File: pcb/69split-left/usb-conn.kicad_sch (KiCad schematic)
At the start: 6 parts, among them J1 USB_C_Receptacle_USB2.0_16P

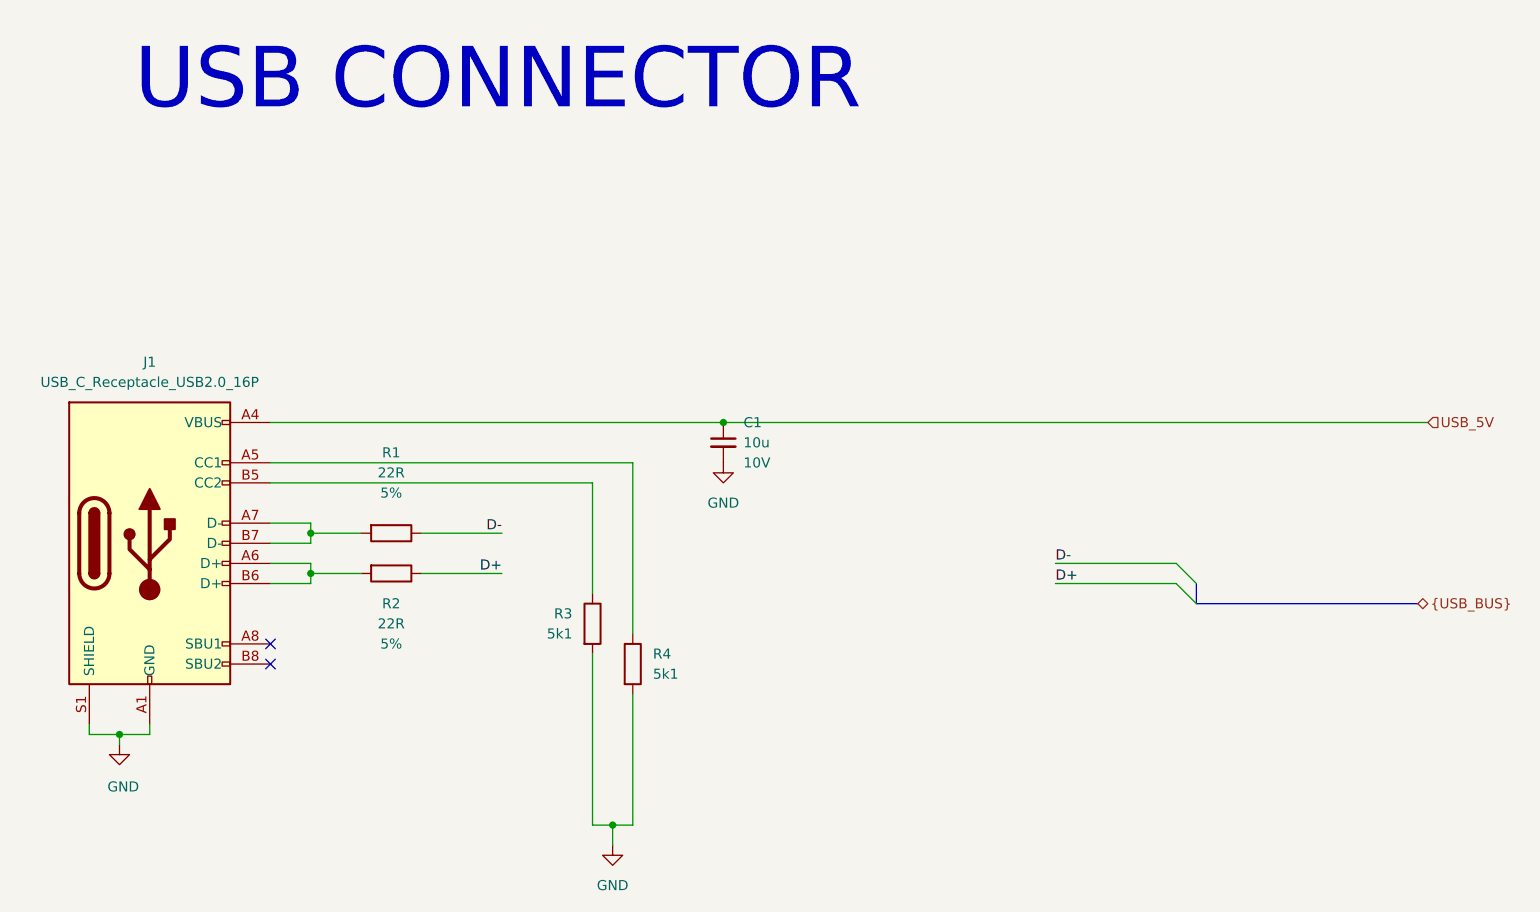
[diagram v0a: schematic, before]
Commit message: Finished left keyboard again...
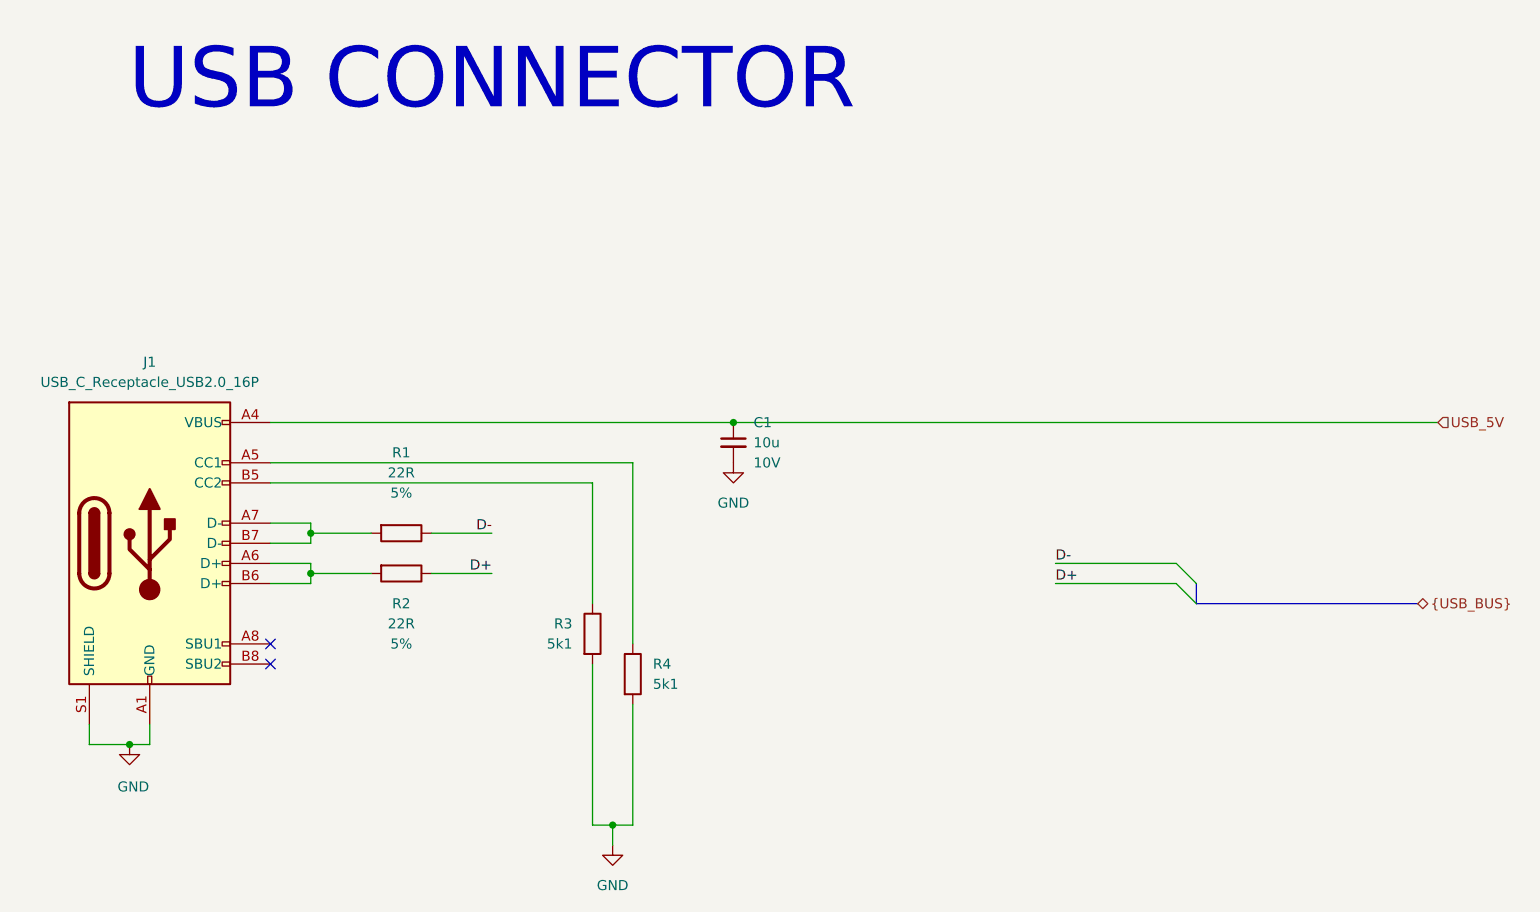
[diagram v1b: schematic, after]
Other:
- moved on the sheet: C1, R1, R2, R3, R4
